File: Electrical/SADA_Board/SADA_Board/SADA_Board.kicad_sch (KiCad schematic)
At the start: 38 parts, among them J1 Headers, J2 Aux. Photodiode Board 1, J3 Aux. Photodiode Board 2, J4 Conn_01x05, J5 Systems Board Connector, U1 STM32L476RGTx, Y1 ECS_Chrystal_

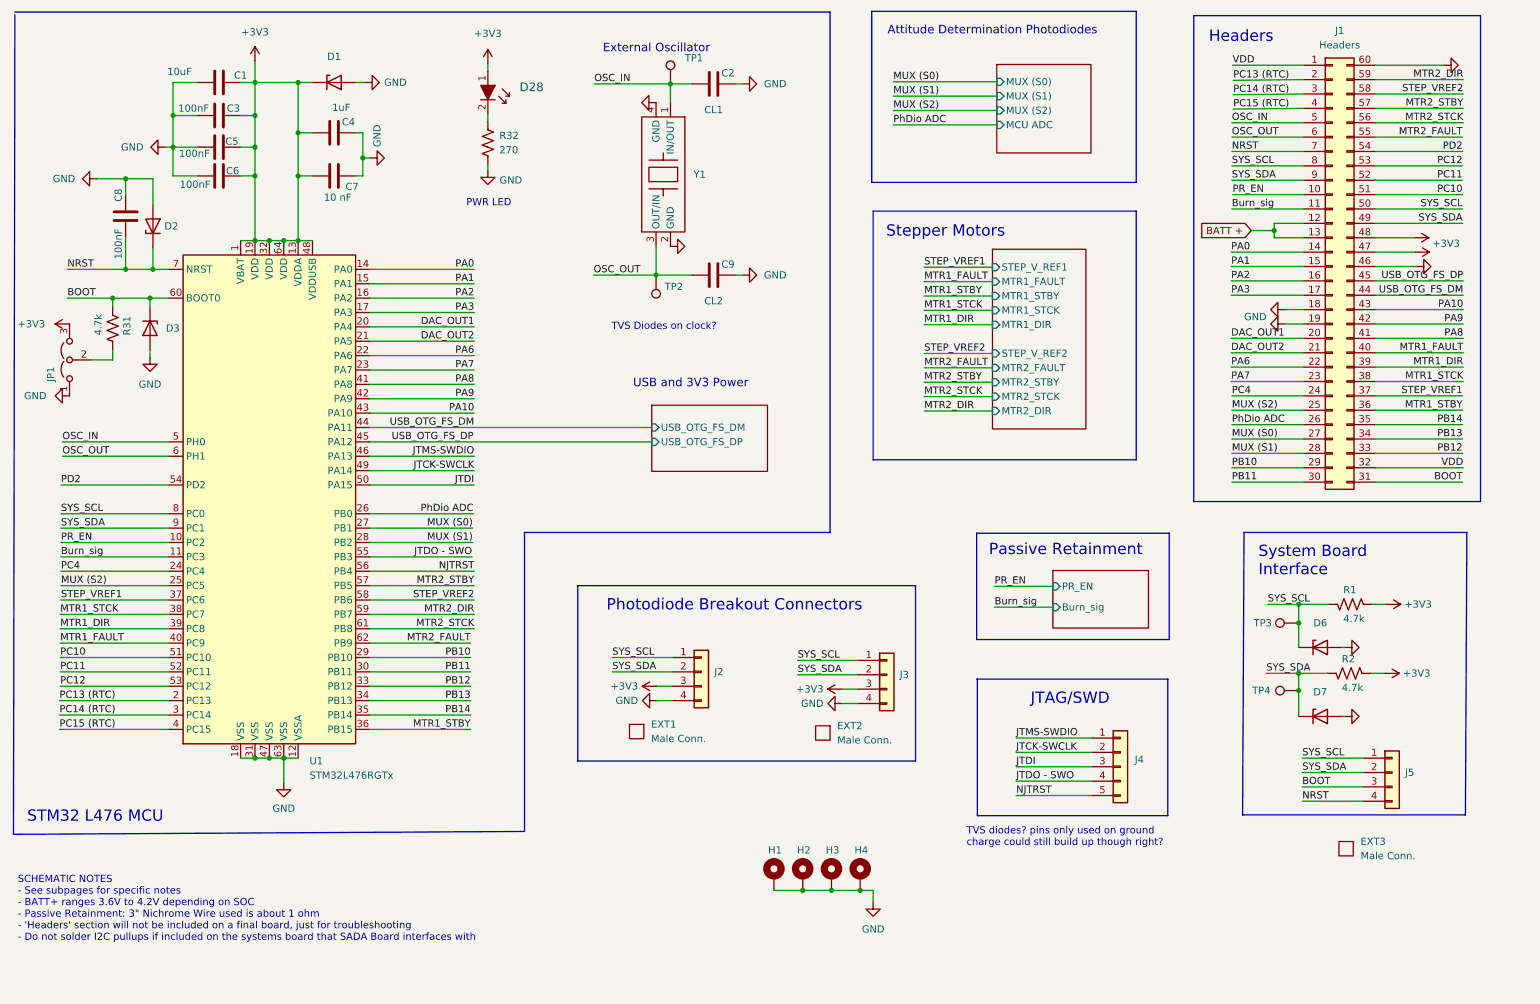
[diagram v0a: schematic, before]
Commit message: Layout rough draft
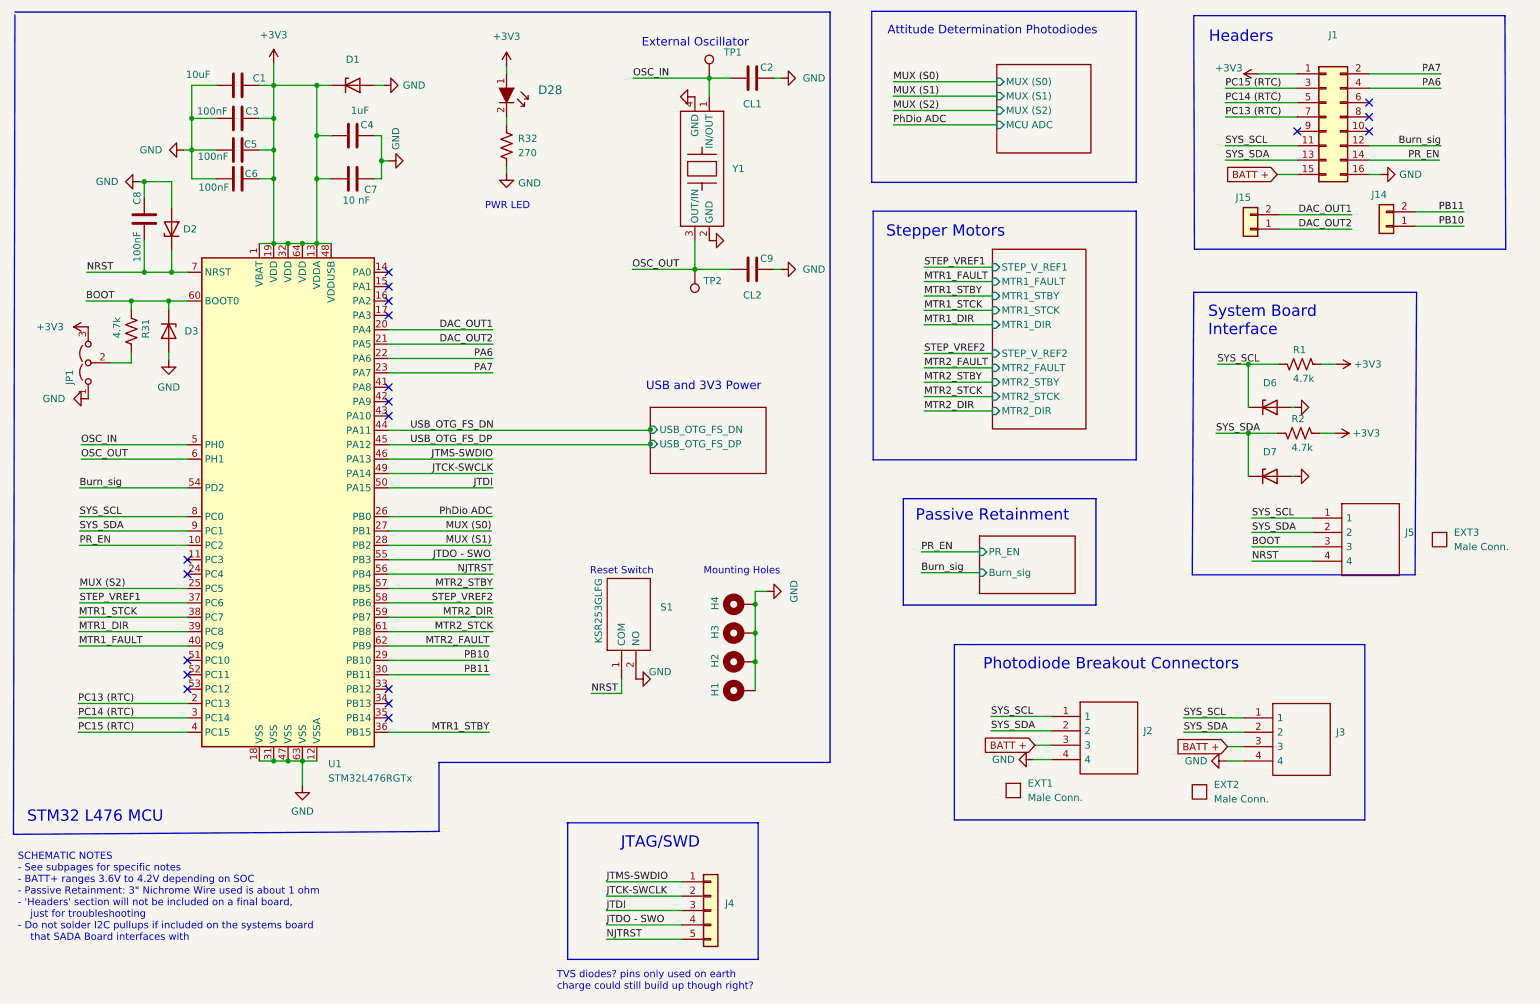
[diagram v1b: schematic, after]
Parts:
- removed J1: Headers, Connector_PinSocket_2.00mm:PinSocket_2x30_P2.00mm_Vertical, symbol Connector_Generic:Conn_02x30_Counter_Clockwise
- removed J2: Aux. Photodiode Board 1, Miles Added:1719730004, symbol Connector_Generic:Conn_01x04
- removed J3: Aux. Photodiode Board 2, Miles Added:1719730004, symbol Connector_Generic:Conn_01x04
- removed J5: Systems Board Connector, Miles Added:1719730004, symbol Connector_Generic:Conn_01x04
- removed TP3, TP4: TestPoint, TestPoint:TestPoint_Pad_D1.0mm, symbol Connector:TestPoint
- added J1: Conn_02x08_Odd_Even, Connector_PinHeader_2.00mm:PinHeader_2x08_P2.00mm_Vertical, symbol Connector_Generic:Conn_02x08_Odd_Even
- added J14, J15: Conn_01x02, Connector_PinSocket_2.00mm:PinSocket_1x02_P2.00mm_Vertical, symbol Connector_Generic:Conn_01x02
- added J2, J3, J5: 70543-0108, SHDR4W64P0X254_1X4_1271X508X1181P, symbol 70543-0108:70543-0108
- added S1: KSR253GLFG, KSR253GLFG, symbol KSR253GLFG:KSR253GLFG
- JP1: footprint Connector_PinHeader_2.00mm:PinHeader_1x03_P2.00mm_Vertical_SMD_Pin1Left -> Connector_PinHeader_2.00mm:PinHeader_1x03_P2.00mm_Vertical
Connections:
- net PD2 is gone; now on net Burn_sig: U1.54 (PD2)
- net +3V3: now also J1.1 (Pin_1)
- net BATT +: now also J1.15 (Pin_15), J2.3, J3.3
- net BOOT: now also J5.3
- net Burn_sig: now also J1.12 (Pin_12); no longer U1.11 (PC3)
- net DAC_OUT1: now also J15.2 (Pin_2)
- net DAC_OUT2: now also J15.1 (Pin_1)
- net GND: now also J1.16 (Pin_16), J2.4, J3.4, S1.2 (NO)
- net NRST: now also J5.4, S1.1 (COM)
- net PA6: now also J1.4 (Pin_4)
- net PA7: now also J1.2 (Pin_2)
- net PB10: now also J14.1 (Pin_1)
- net PB11: now also J14.2 (Pin_2)
- net PC13 (RTC): now also J1.7 (Pin_7)
- net PC14 (RTC): now also J1.5 (Pin_5)
- net PC15 (RTC): now also J1.3 (Pin_3)
- net PR_EN: now also J1.14 (Pin_14)
- net SYS_SCL: now also J1.11 (Pin_11), J2.1, J3.1, J5.1
- net SYS_SDA: now also J1.13 (Pin_13), J2.2, J3.2, J5.2
- net PA0: no longer names the net of U1.14 (PA0)
- net PA1: no longer names the net of U1.15 (PA1)
- net PA10: no longer names the net of U1.43 (PA10)
- net PA2: no longer names the net of U1.16 (PA2)
- net PA3: no longer names the net of U1.17 (PA3)
- net PA8: no longer names the net of U1.41 (PA8)
- net PA9: no longer names the net of U1.42 (PA9)
- net PB12: no longer names the net of U1.33 (PB12)
- net PB13: no longer names the net of U1.34 (PB13)
- net PB14: no longer names the net of U1.35 (PB14)
- net PC10: no longer names the net of U1.51 (PC10)
- net PC11: no longer names the net of U1.52 (PC11)
- net PC12: no longer names the net of U1.53 (PC12)
- net PC4: no longer names the net of U1.24 (PC4)
- net USB_OTG_FS_DM renamed USB_OTG_FS_DN
- no-connect marks 0 -> 19
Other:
- sheet USB and MCU LDO ports: added USB_OTG_FS_DN; removed USB_OTG_FS_DM
- note added: "Mounting Holes"
- note added: "Reset Switch"
- note added: "TVS diodes? pins only used on earth charge could still build up though right?"
- note removed: "TVS Diodes on clock?"
- note removed: "TVS diodes? pins only used on ground charge could still build up though right?"
- moved on the sheet: C1, C2, C3, C4, C5, C6, C7, C8, C9, D1, D2, D28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
